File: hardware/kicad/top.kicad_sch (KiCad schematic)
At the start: 0 parts

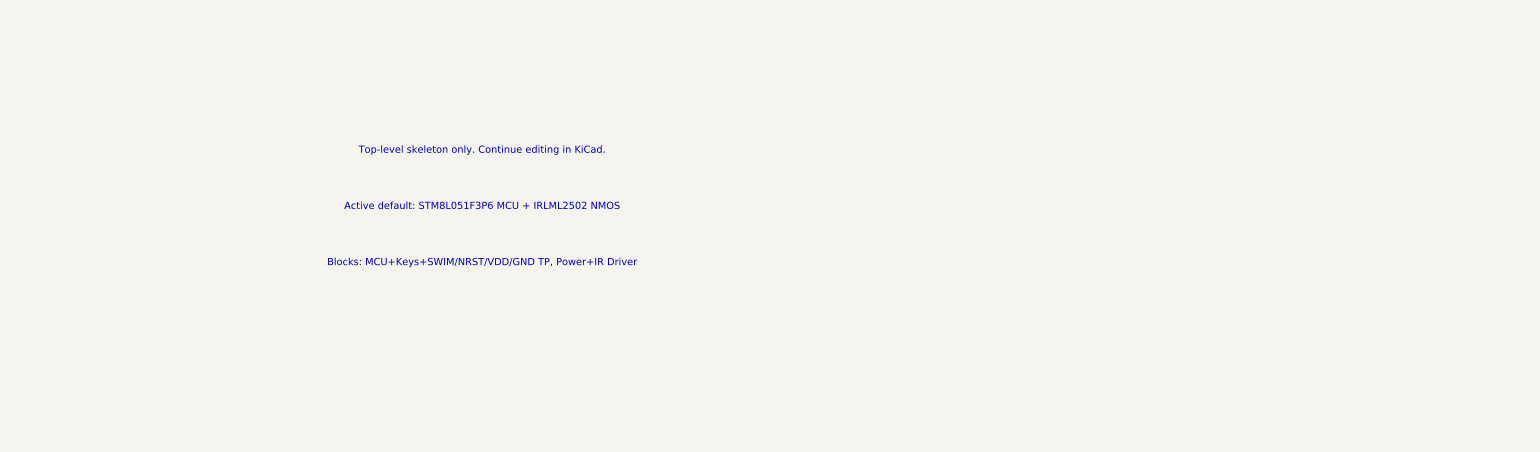
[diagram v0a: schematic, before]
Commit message: sch opt
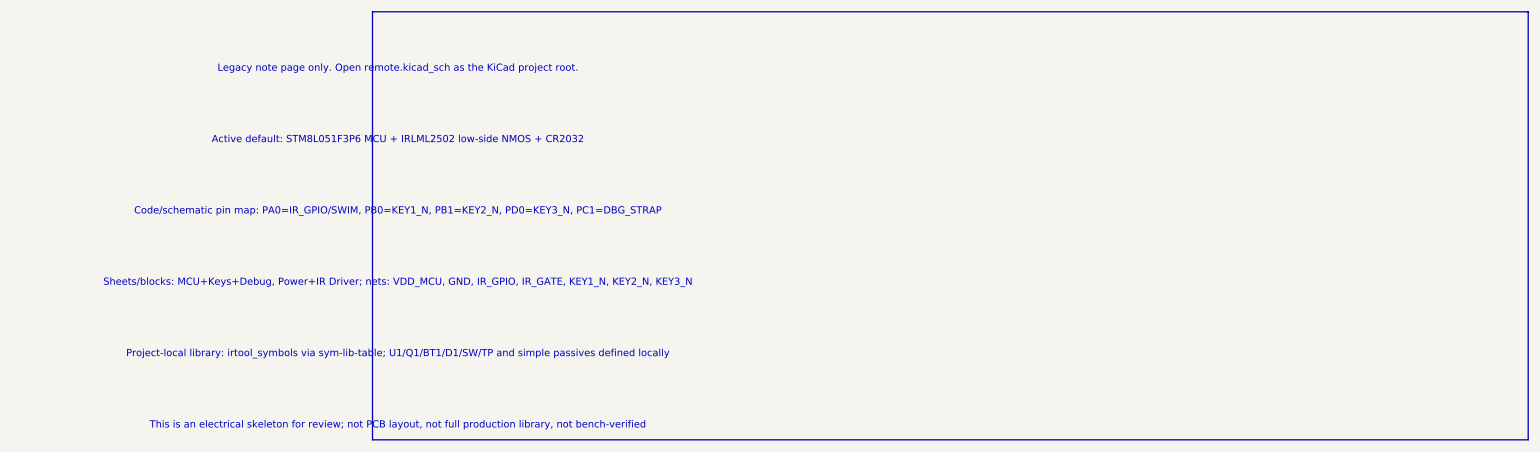
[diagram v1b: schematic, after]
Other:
- note added: "Active default: STM8L051F3P6 MCU + IRLML2502 low-side NMOS + CR2032"
- note added: "Code/schematic pin map: PA0=IR_GPIO/SWIM, PB0=KEY1_N, PB1=KEY2_N, PD0=KEY3_N, PC1=DBG_STRAP"
- note added: "Legacy note page only. Open remote.kicad_sch as the KiCad project root."
- note added: "Project-local library: irtool_symbols via sym-lib-table; U1/Q1/BT1/D1/SW/TP and simple passives defined locally"
- note added: "Sheets/blocks: MCU+Keys+Debug, Power+IR Driver; nets: VDD_MCU, GND, IR_GPIO, IR_GATE, KEY1_N, KEY2_N, KEY3_N"
- note added: "This is an electrical skeleton for review; not PCB layout, not full production library, not bench-verified"
- note removed: "Active default: STM8L051F3P6 MCU + IRLML2502 NMOS"
- note removed: "Blocks: MCU+Keys+SWIM/NRST/VDD/GND TP, Power+IR Driver"
- note removed: "Top-level skeleton only. Continue editing in KiCad."
- title: STM8L051F3P6 IRLML2502 CR2032 NEC Remote - Skeleton -> STM8L051F3P6 IRLML2502 CR2032 NEC Remote - Electrical Skeleton
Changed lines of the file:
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@@
 (kicad_sch (version 20230121) (generator "codex")
   (paper "A4")
-  (title_block (title "STM8L051F3P6 IRLML2502 CR2032 NEC Remote - Skeleton"))
-  (text "Top-level skeleton only. Continue editing in KiCad." (at 50 40 0) (effects (font (size 1.27 1.27))))
-  (text "Active default: STM8L051F3P6 MCU + IRLML2502 NMOS" (at 50 50 0) (effects (font (size 1.27 1.27))))
-  (text "Blocks: MCU+Keys+SWIM/NRST/VDD/GND TP, Power+IR Driver" (at 50 60 0) (effects (font (size 1.27 1.27))))
+  (title_block (title "STM8L051F3P6 IRLML2502 CR2032 NEC Remote - Electrical Skeleton"))
+  (polyline
+    (pts (xy 30.48 15.24) (xy 236.22 15.24) (xy 236.22 91.44) (xy 30.48 91.44) (xy 30.48 15.24))
+    (stroke (width 0.2) (type default) (color 0 0 0 0))
+  )
+  (text "Legacy note page only. Open remote.kicad_sch as the KiCad project root." (at 35 25.4 0) (effects (font (size 1.27 1.27))))
+  (text "Active default: STM8L051F3P6 MCU + IRLML2502 low-side NMOS + CR2032" (at 35 38.1 0) (effects (font (size 1.27 1.27))))
+  (text "Code/schematic pin map: PA0=IR_GPIO/SWIM, PB0=KEY1_N, PB1=KEY2_N, PD0=KEY3_N, PC1=DBG_STRAP" (at 35 50.8 0) (effects (font (size 1.27 1.27))))
+  (text "Sheets/blocks: MCU+Keys+Debug, Power+IR Driver; nets: VDD_MCU, GND, IR_GPIO, IR_GATE, KEY1_N, KEY2_N, KEY3_N" (at 35 63.5 0) (effects (font (size 1.27 1.27))))
+  (text "Project-local library: irtool_symbols via sym-lib-table; U1/Q1/BT1/D1/SW/TP and simple passives defined locally" (at 35 76.2 0) (effects (font (size 1.27 1.27))))
+  (text "This is an electrical skeleton for review; not PCB layout, not full production library, not bench-verified" (at 35 88.9 0) (effects (font (size 1.27 1.27))))
+  (path "/" (page "99"))
 )
